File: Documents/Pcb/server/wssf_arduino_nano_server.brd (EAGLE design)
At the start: 54 x 38 mm, 10 parts

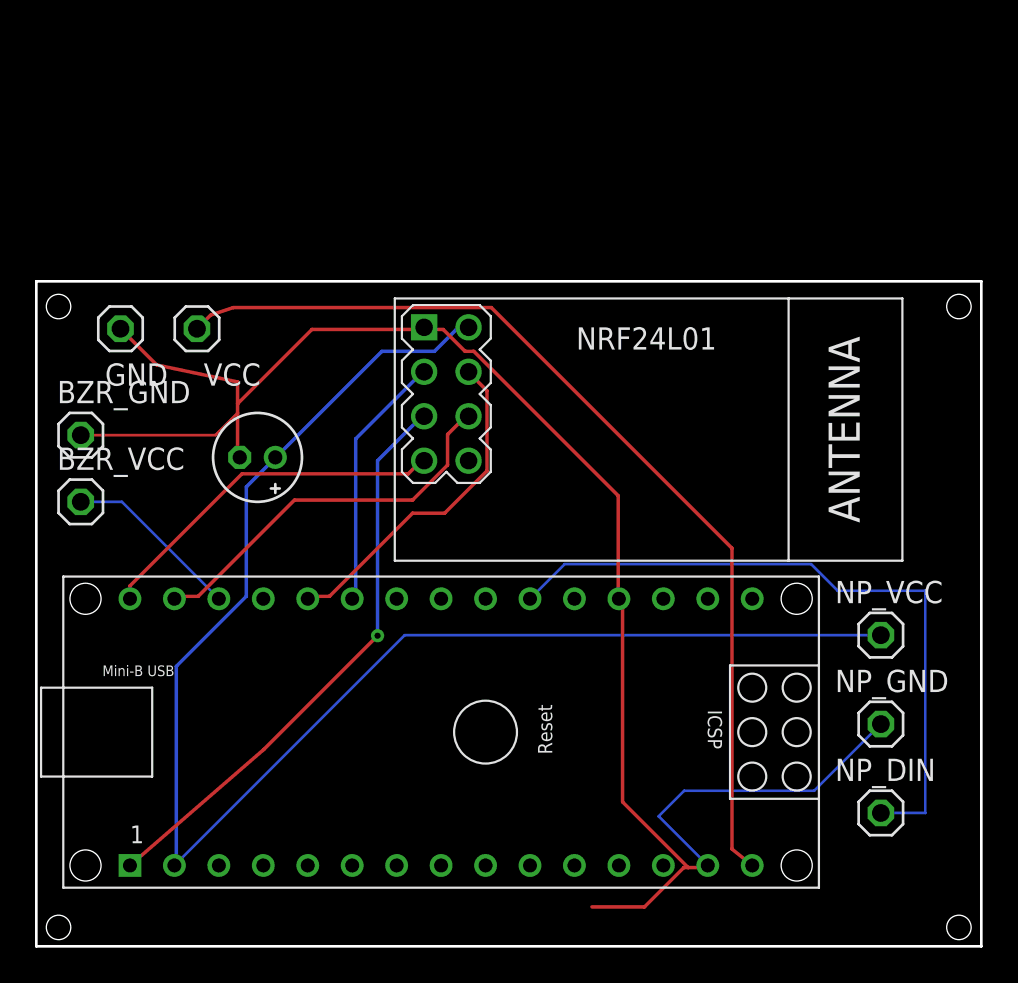
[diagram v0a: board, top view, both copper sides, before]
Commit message: update pcbs and add gerbers files
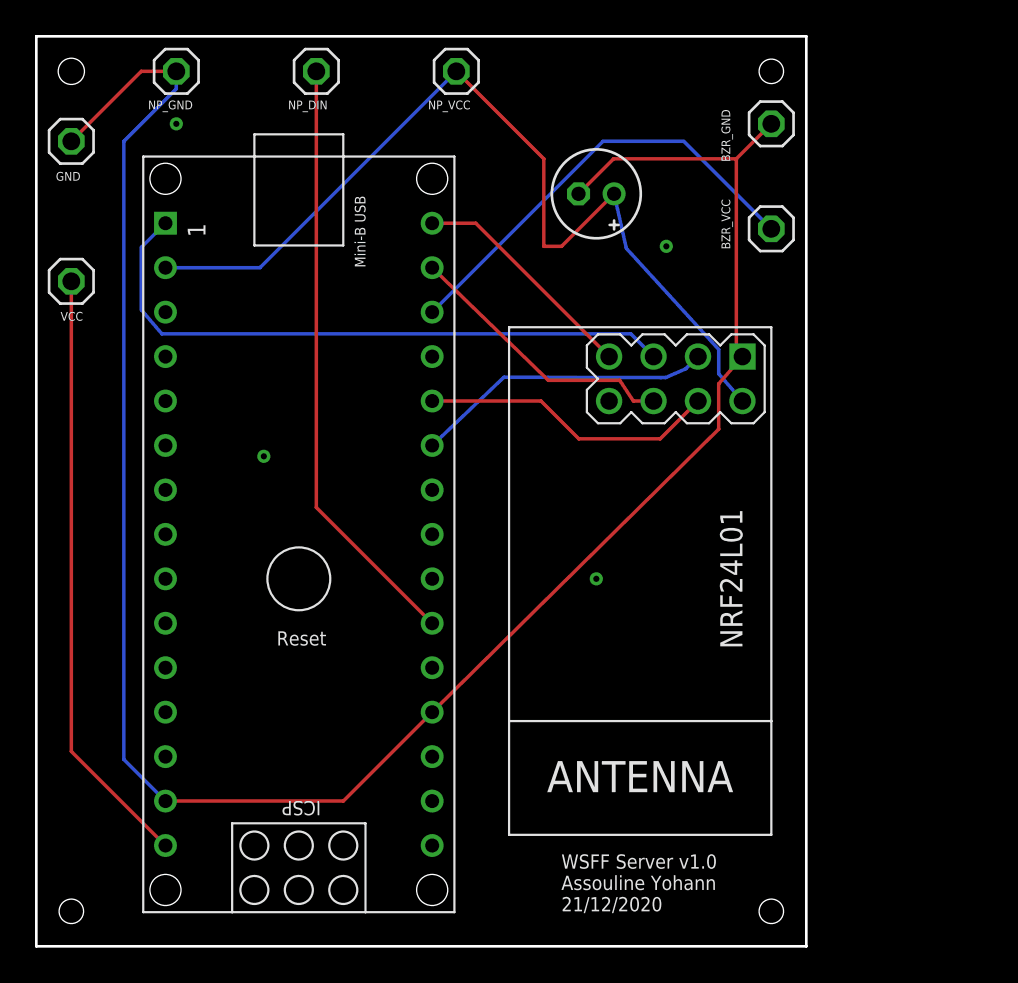
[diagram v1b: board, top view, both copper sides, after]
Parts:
- moved NP_GND 54.9 mm to (8.00, 50.0)
- moved NP_DIN 53.3 mm to (16.0, 50.0)
- moved BZR_GND 43.3 mm to (42.0, 47.0)
- moved BZR_VCC 42.4 mm to (42.0, 41.0)
- moved NP_VCC 40.3 mm to (24.0, 50.0)
- moved C1 24.5 mm to (32.0, 43.0)
- moved ARDUINO_NANO1 13.8 mm to (15.0, 21.0), turned to 270 degrees
- moved GND 11.1 mm to (2.00, 46.0)
- moved NRF24L01 8.07 mm to (34.0, 21.0), turned to 270 degrees
- moved VCC 7.67 mm to (2.00, 38.0)
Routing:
- net VCC: track 85.6 -> 53.1 mm
- net GND: track 98.5 -> 120.7 mm, vias 0 -> 4
- net VCC_IN: track 55.3 -> 34.5 mm
- net BZR_DIN: track 10.2 -> 25.5 mm
- net MISO_NRF: track 20.5 -> 13.3 mm
- net MOSI_NRF: track 22.2 -> 15.9 mm
- net NEOPIXEL_DIN: track 39.3 -> 34.3 mm
- net SCK_NRF: track 33.0 -> 36.0 mm, vias 1 -> 0
- net CE_NRF: track 14.7 -> 17.1 mm
- net CSN_NRF: track 19.3 -> 17.0 mm
- added copper zone on layer 1, net GND
- added copper zone on layer 16, net GND
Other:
- board size 54 x 38 mm -> 44 x 52 mm
- board text added: "WSFF Server v1.0 Assouline Yohann 21/12/2020"
